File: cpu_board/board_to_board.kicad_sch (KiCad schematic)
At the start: 2 parts

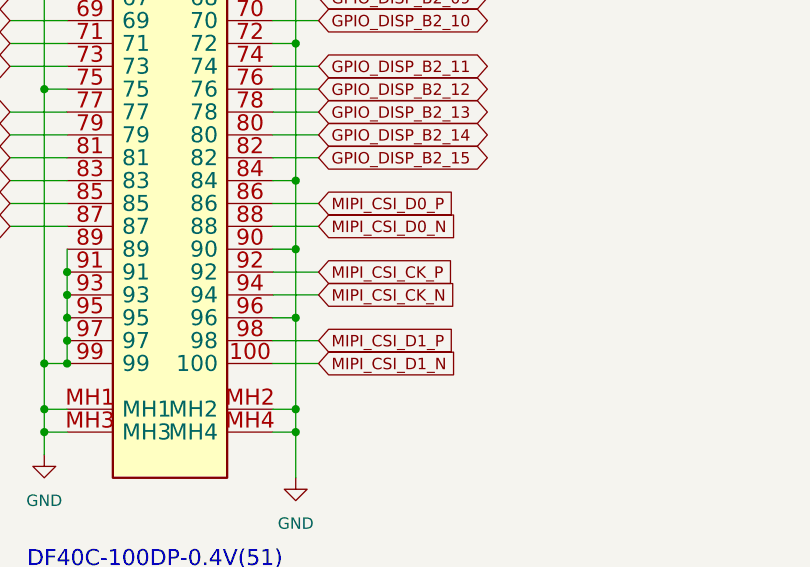
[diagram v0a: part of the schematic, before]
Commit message: pre-autorouter
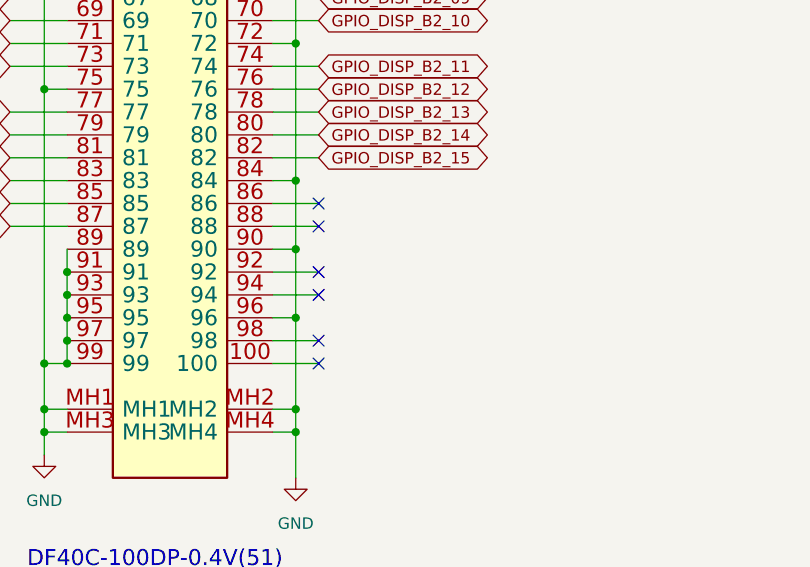
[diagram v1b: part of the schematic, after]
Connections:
- net MIPI_CSI_CK_N: no longer names the net of J?.94
- net MIPI_CSI_CK_P: no longer names the net of J?.92
- net MIPI_CSI_D0_N: no longer names the net of J?.88
- net MIPI_CSI_D0_P: no longer names the net of J?.86
- net MIPI_CSI_D1_N: no longer names the net of J?.100
- net MIPI_CSI_D1_P: no longer names the net of J?.98
- no-connect marks 9 -> 15
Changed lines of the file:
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@@
   )
   (no_connect (at 129.54 171.45))
+  (no_connect (at 313.055 206.375))
   (no_connect (at 129.54 184.15))
   (no_connect (at 129.54 186.69))
+  (no_connect (at 313.055 196.215))
   (no_connect (at 129.54 176.53))
   (no_connect (at 129.54 153.67))
   (no_connect (at 129.54 173.99))
+  (no_connect (at 313.055 198.755))
+  (no_connect (at 313.055 203.835))
   (no_connect (at 129.54 191.77))
+  (no_connect (at 313.055 188.595))
   (no_connect (at 129.54 189.23))
+  (no_connect (at 313.055 191.135))
   (no_connect (at 129.54 179.07))
   (wire (pts (xy 307.975 186.055) (xy 310.515 186.055))
@@
     )
   )
-  (global_label "MIPI_CSI_D0_N" (shape input) (at 313.055 191.135 0) (fields_autoplaced)
-    (effects (font (size 1.27 1.27)) (justify left))
-    (property "Intersheetrefs" "${INTERSHEET_REFS}" (at 329.0995 191.135 0)
-      (effects (font (size 1.27 1.27)) (justify left) hide)
-    )
-  )
-  (global_label "MIPI_CSI_D0_P" (shape input) (at 313.055 188.595 0) (fields_autoplaced)
-    (effects (font (size 1.27 1.27)) (justify left))
-    (property "Intersheetrefs" "${INTERSHEET_REFS}" (at 329.0414 188.595 0)
-      (effects (font (size 1.27 1.27)) (justify left) hide)
-    )
-  )
   (global_label "GPIO_EMC_B2_12" (shape bidirectional) (at 278.765 168.275 180)
     (effects (font (size 1.27 1.27)) (justify right))
@@
     )
   )
-  (global_label "MIPI_CSI_CK_P" (shape input) (at 313.055 196.215 0) (fields_autoplaced)
-    (effects (font (size 1.27 1.27)) (justify left))
-    (property "Intersheetrefs" "${INTERSHEET_REFS}" (at 329.0995 196.215 0)
-      (effects (font (size 1.27 1.27)) (justify left) hide)
-    )
-  )
   (global_label "GPIO_DISP_B2_12" (shape bidirectional) (at 313.055 175.895 0) (fields_autoplaced)
     (effects (font (size 1.27 1.27)) (justify left))
@@
     )
   )
-  (global_label "MIPI_CSI_CK_N" (shape input) (at 313.055 198.755 0) (fields_autoplaced)
-    (effects (font (size 1.27 1.27)) (justify left))
-    (property "Intersheetrefs" "${INTERSHEET_REFS}" (at 329.1576 198.755 0)
-      (effects (font (size 1.27 1.27)) (justify left) hide)
-    )
-  )
   (global_label "GPIO_AD_33" (shape bidirectional) (at 129.54 201.93 0) (fields_autoplaced)
     (effects (font (size 1.27 1.27)) (justify left))
@@
     )
   )
-  (global_label "MIPI_CSI_D1_P" (shape input) (at 313.055 203.835 0) (fields_autoplaced)
-    (effects (font (size 1.27 1.27)) (justify left))
-    (property "Intersheetrefs" "${INTERSHEET_REFS}" (at 329.0414 203.835 0)
-      (effects (font (size 1.27 1.27)) (justify left) hide)
-    )
-  )
   (global_label "GPIO_SNVS_09" (shape input) (at 278.765 127.635 180) (fields_autoplaced)
     (effects (font (size 1.27 1.27)) (justify right))
@@
     )
   )
-  (global_label "MIPI_CSI_D1_N" (shape input) (at 313.055 206.375 0) (fields_autoplaced)
-    (effects (font (size 1.27 1.27)) (justify left))
-    (property "Intersheetrefs" "${INTERSHEET_REFS}" (at 329.0995 206.375 0)
-      (effects (font (size 1.27 1.27)) (justify left) hide)
-    )
-  )
